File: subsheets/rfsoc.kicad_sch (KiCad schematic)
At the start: 27 parts, among them U1 nRF54L15-QFXX, U2 ADXL367BCCZ-RL7, X2 32MHz

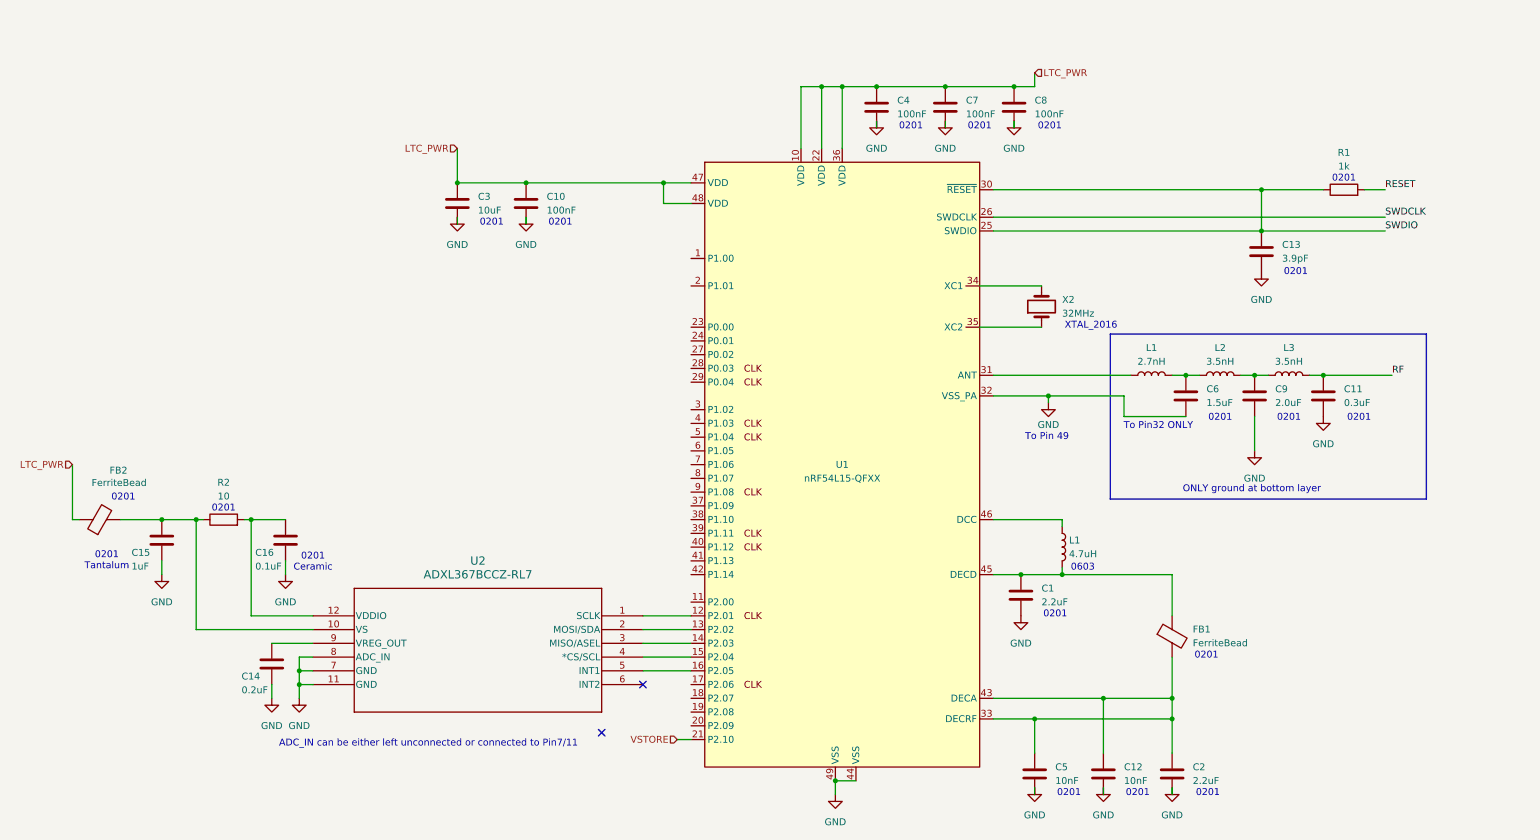
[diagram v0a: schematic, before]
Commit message: Finished Schematic
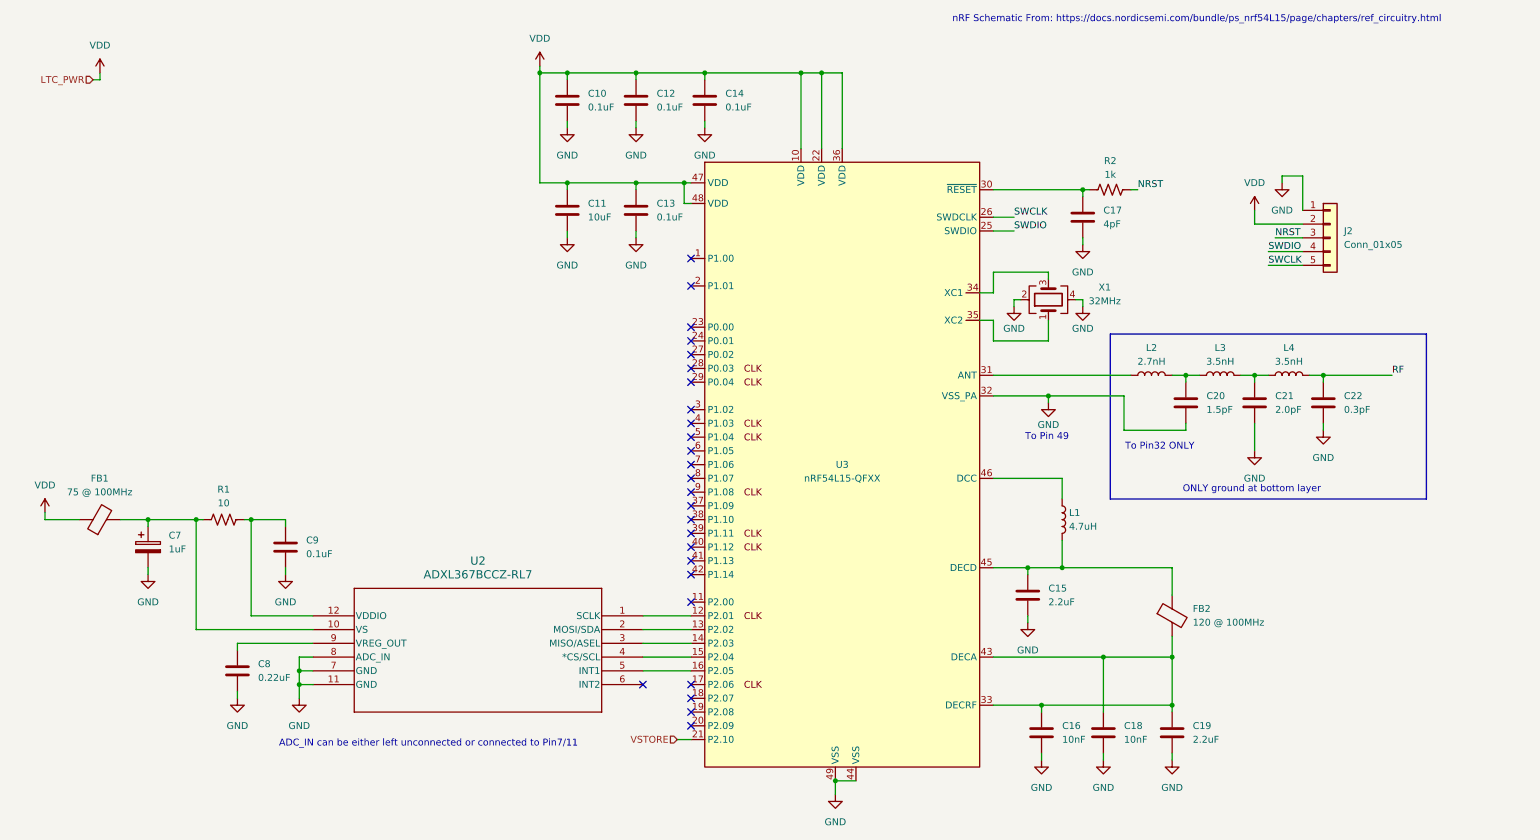
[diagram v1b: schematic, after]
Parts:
- removed C1: 2.2uF, symbol Device:C
- removed C2: 2.2uF, 0603, symbol Device:C
- removed C4, C7: 100nF, 0603, symbol Device:C
- removed C5: 10nF, 0603, symbol Device:C
- removed FB2: FerriteBead, symbol Device:FerriteBead
- removed L3: 3.5nH, symbol Device:L
- removed R1: 1k, symbol Device:R
- added C13, C9: 0.1uF, Capacitor_SMD:C_0603_1608Metric, symbol Device:C
- added C18: 10nF, Capacitor_SMD:C_0603_1608Metric, symbol Device:C
- added C19: 2.2uF, Capacitor_SMD:C_0603_1608Metric, symbol Device:C
- added C7: 1uF, Capacitor_SMD:C_0603_1608Metric_Pad1.08x0.95mm_HandSolder, symbol Device:C_Polarized
- added FB1: 75 @ 100MHz, Inductor_SMD:L_0603_1608Metric, symbol Device:FerriteBead
- added J2: Conn_01x05, Connector_PinHeader_1.00mm:PinHeader_1x05_P1.00mm_Vertical, symbol Connector_Generic:Conn_01x05
- added L4: 3.5nH, Inductor_SMD:L_0201_0603Metric, symbol Device:L
- added R2: 1k, Resistor_SMD:R_0603_1608Metric_Pad0.98x0.95mm_HandSolder, symbol Device:R_US
- C10: value 100nF -> 0.1uF; footprint 0603 -> Capacitor_SMD:C_0603_1608Metric; Part (none) -> CL10B104KB8NNNC; Tolerance (none) -> 10%; Voltage (none) -> 50V
- C11: renamed from C3; footprint 0603 -> Capacitor_SMD:C_0603_1608Metric; Part (none) -> CL10A106KQ8NNNC; Tolerance (none) -> 10%; Voltage (none) -> 6.3V
- C12: value 10nF -> 0.1uF; footprint 0603 -> Capacitor_SMD:C_0603_1608Metric; Part (none) -> CL10B104KB8NNNC; Tolerance (none) -> 10%; Voltage (none) -> 50V
- C14: value 0.2uF -> 0.1uF; footprint (none) -> Capacitor_SMD:C_0603_1608Metric; Part (none) -> CL10B104KB8NNNC; Tolerance (none) -> 10%; Voltage (none) -> 50V
- C15: value 1uF -> 2.2uF; footprint (none) -> Capacitor_SMD:C_0603_1608Metric; Part (none) -> CL10A225KO8NNNC; Tolerance (none) -> 10%; Voltage (none) -> 16V
- C16: value 0.1uF -> 10nF; footprint (none) -> Capacitor_SMD:C_0603_1608Metric; Part (none) -> CL10B103KB8NNNC; Tolerance (none) -> 10%; Voltage (none) -> 50V
- C17: renamed from C13; value 3.9pF -> 4pF; footprint (none) -> Capacitor_SMD:C_0603_1608Metric; Part (none) -> CL10C040CB8NNNC; Tolerance (none) -> 6.25%; Voltage (none) -> 50V
- C20: renamed from C6; value 1.5uF -> 1.5pF; footprint 0603 -> Capacitor_SMD:C_0201_0603Metric; Part (none) -> GJM0335C1E1R5WB01D
- C21: renamed from C9; value 2.0uF -> 2.0pF; footprint 0603 -> Capacitor_SMD:C_0201_0603Metric; Part (none) -> GJM0335C1E2R0WB01D
- C22: renamed from C11; value 0.3uF -> 0.3pF; footprint 0603 -> Capacitor_SMD:C_0201_0603Metric; Part (none) -> GJM0335C1ER30WB01D
- C8: value 100nF -> 0.22uF; footprint 0603 -> Capacitor_SMD:C_0603_1608Metric; Part (none) -> CL10B224KO8NNNC; Tolerance (none) -> 10%; Voltage (none) -> 16V
- FB2: renamed from FB1; value FerriteBead -> 120 @ 100MHz; footprint (none) -> Inductor_SMD:L_0603_1608Metric; Part (none) -> BLM18KG121TN1D
- L1: footprint (none) -> Inductor_SMD:L_0603_1608Metric; Current (none) -> 620mA; Part (none) -> LQM18PN4R7MFRL; Tolerance (none) -> 20%
- L2: renamed from L1; footprint (none) -> Inductor_SMD:L_0201_0603Metric; Part (none) -> LQP03HQ2N7B02D
- L3: renamed from L2; footprint (none) -> Inductor_SMD:L_0201_0603Metric; Part (none) -> LQP03HQ3N5B02D
- R1: renamed from R2; footprint (none) -> Resistor_SMD:R_0603_1608Metric; symbol Device:R -> Device:R_US; Part (none) -> ERJ-3EKF10R0V; Tolerance (none) -> 1%; Wattage (none) -> 1/10W
- U2: footprint (none) -> earworm:LGA-CC-12-4
- X1: renamed from X2; footprint (none) -> Crystal:Crystal_SMD_2016-4Pin_2.0x1.6mm; symbol Device:Crystal -> Device:Crystal_GND24; Part (none) -> ECS-320-8-37CKM; Stability (none) -> 10ppm; lc (none) -> 8pF
- renumbered U1 to U3
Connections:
- net GND: now also X1.2, X1.4, C13.2, C18.2, C19.2, C7.2, C9.2, J2.1 (Pin_1)
- net RF: now also L4.2
- net SWDIO: now also J2.4 (Pin_4); no longer C17.1, U3.30 (~{RESET})
- net at R1.2, U2.12 (VDDIO): now also C9.1; no longer C16.1
- net at U2.9 (VREG_OUT): now also C8.1; no longer C14.1
- net at R1.1, U2.10 (VS): now also C7.1, FB1.2; no longer C15.1
- net at FB2.2, U3.33 (DECRF), U3.43 (DECA): now also C16.1, C18.1, C19.1; no longer C12.1
- net at C21.1, L3.2: now also L4.1
- net at FB2.1, L1.2, U3.45 (DECD): now also C15.1
- net at U3.34 (XC1): now also X1.3; no longer X1.2
- net LTC_PWR renamed VDD
- net VDD: now also C12.1, C14.1, C13.1, FB1.1, J2.2 (Pin_2); no longer C8.1
- net SWDCLK renamed SWCLK
- net SWCLK: now also J2.5 (Pin_5)
- new net: C17.1, R2.1, U3.30 (~{RESET})
- new net NRST: J2.3 (Pin_3), R2.2
- no-connect marks 2 -> 26
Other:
- note added: "nRF Schematic From: https://docs.nordicsemi.com/bundle/ps_nrf54L15/page/chapters/ref_circuitry.html"
- note removed: "0201"
- note removed: "0201 Ceramic"
- note removed: "0201 Tantalum"
- note removed: "0603"
- note removed: "XTAL_2016"
- moved on the sheet: C11, C17, C20, C21, C22, FB2, L1
